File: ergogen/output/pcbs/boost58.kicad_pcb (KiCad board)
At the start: 2 copper layers, 147.5 x 127.5 mm, 110 parts, among them SW1 %R, SW10 %R, SW11 %R, SW12 %R, SW13 %R, SW14 %R, SW15 %R, SW16 %R, SW17 %R, SW18 %R, SW19 %R, SW2 %R, SW20 %R, SW21 %R, SW22 %R, SW23 %R, SW24 %R, SW25 %R, SW26 %R, SW27 %R, SW28 %R, SW29 %R, SW3 %R, SW4 %R, SW5 %R, SW6 %R, SW7 %R, SW8 %R, SW9 %R

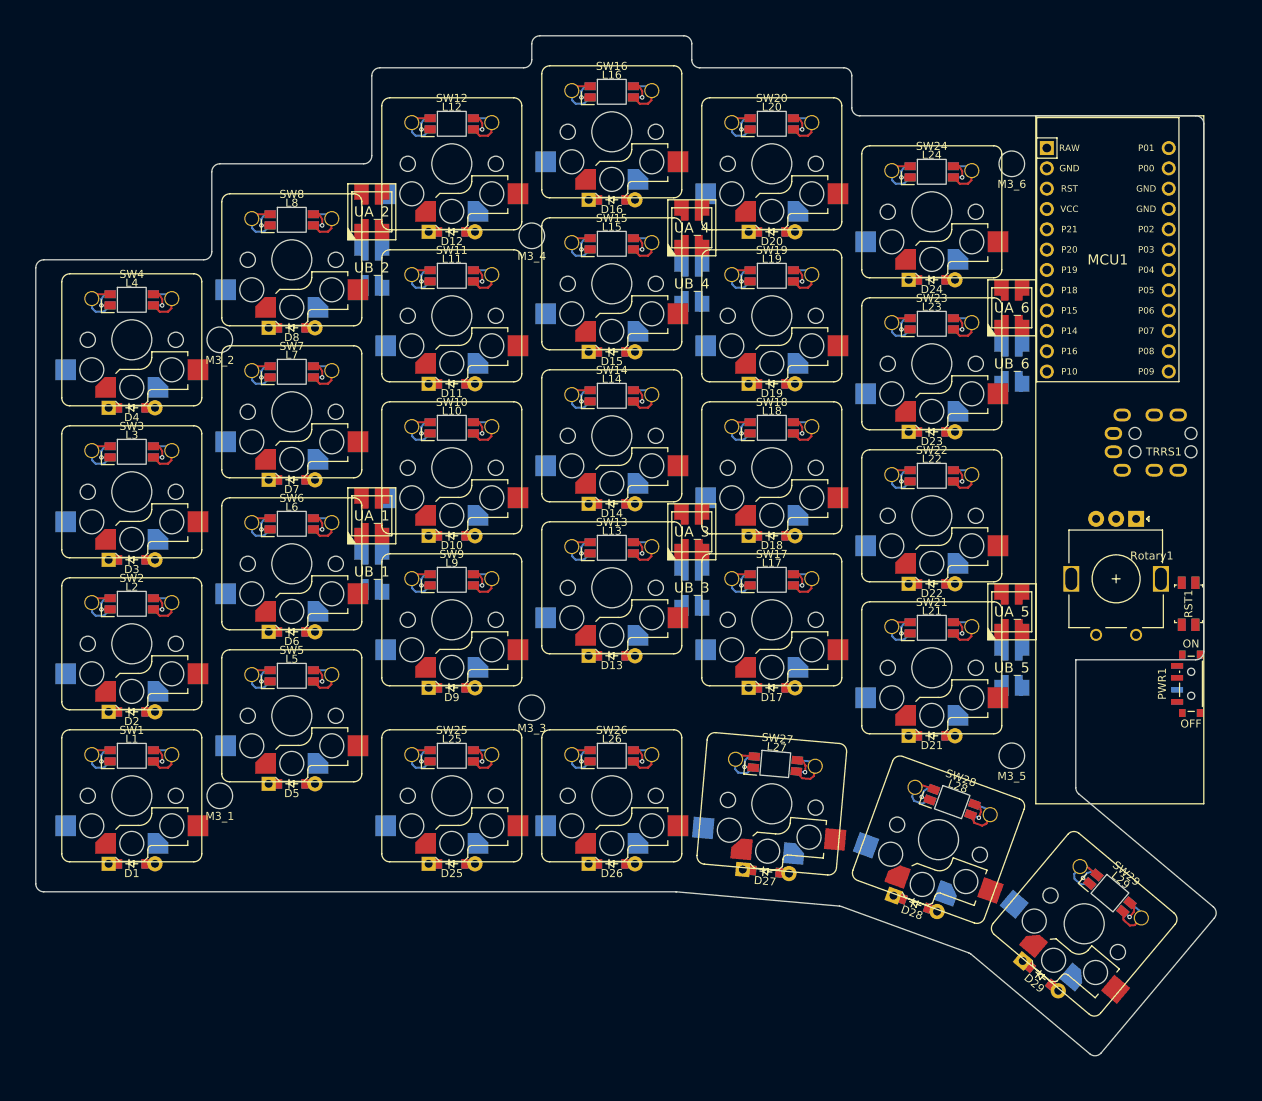
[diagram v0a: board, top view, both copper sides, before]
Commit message: re-generated drawings and PCB
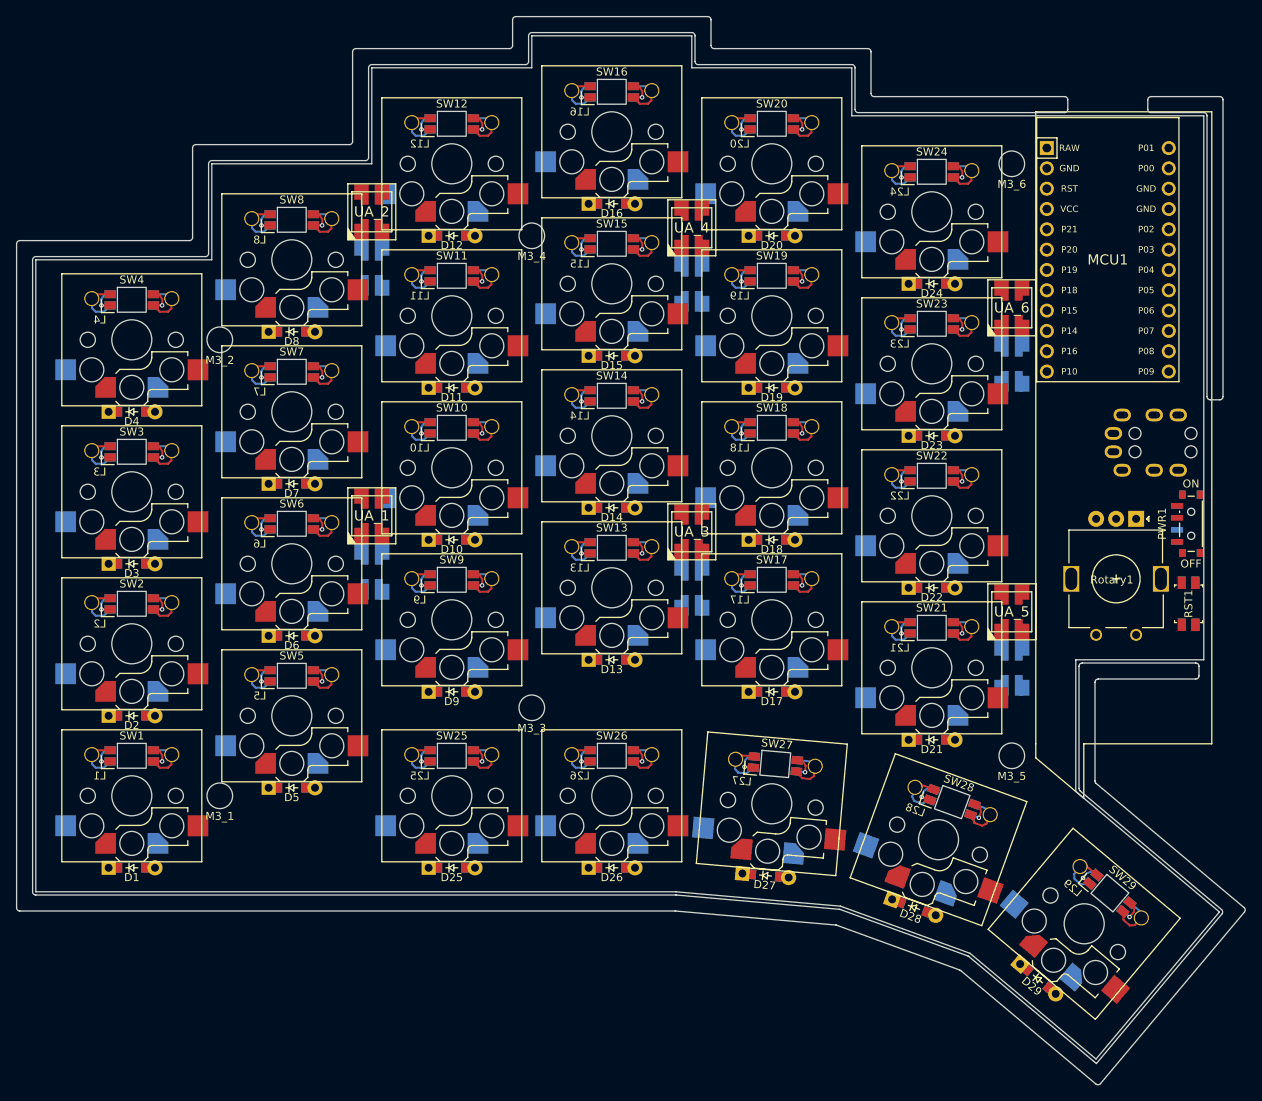
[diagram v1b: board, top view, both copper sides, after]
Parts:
- moved PWR1 20.0 mm to (172.4, 86.0)
- moved D27 0.50 mm to (119.2, 130.0)
- moved D1 0.50 mm to (40.0, 129.0)
- moved D10 0.50 mm to (80.0, 88.0)
- moved D11 0.50 mm to (80.0, 69.0)
- moved D12 0.50 mm to (80.0, 50.0)
- moved D13 0.50 mm to (100.0, 103.0)
- moved D14 0.50 mm to (100.0, 84.0)
- moved D15 0.50 mm to (100.0, 65.0)
- moved D16 0.50 mm to (100.0, 46.0)
- moved D17 0.50 mm to (120.0, 107.0)
- moved D18 0.50 mm to (120.0, 88.0)
- moved D19 0.50 mm to (120.0, 69.0)
- moved D2 0.50 mm to (40.0, 110.0)
- moved D20 0.50 mm to (120.0, 50.0)
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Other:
- board size 147.5 x 127.5 mm -> 153.6 x 133.5 mm
